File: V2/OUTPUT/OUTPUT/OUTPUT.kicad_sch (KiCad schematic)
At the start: 32 parts, among them J1 Conn_01x03, J2 Conn_01x03, J3 Conn_01x03, J4 Conn_01x03, J5 Conn_01x03, J6 Conn_01x03, J7 Conn_01x03, J8 Conn_01x03, Q1 QM6006D, Q2 QM6006D, Q3 QM6006D, Q4 QM6006D, Q5 QM6006D, Q6 QM6006D, Q7 QM6006D, Q8 QM6006D

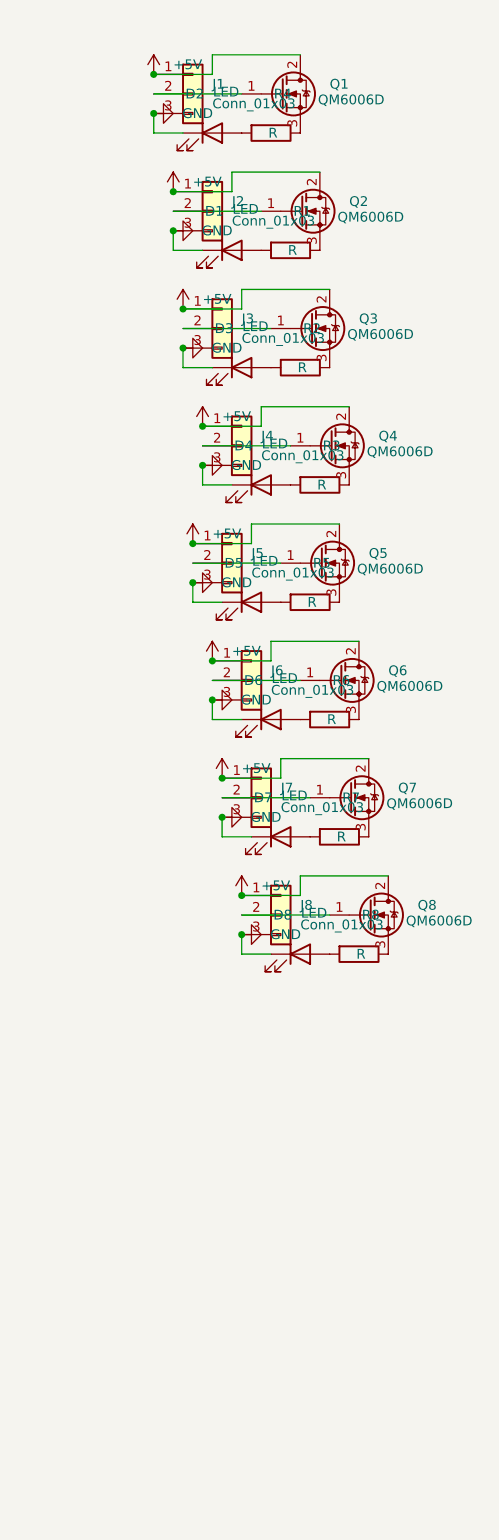
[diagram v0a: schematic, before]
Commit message: Auto-update: 28.03.2026 23:45:51,95
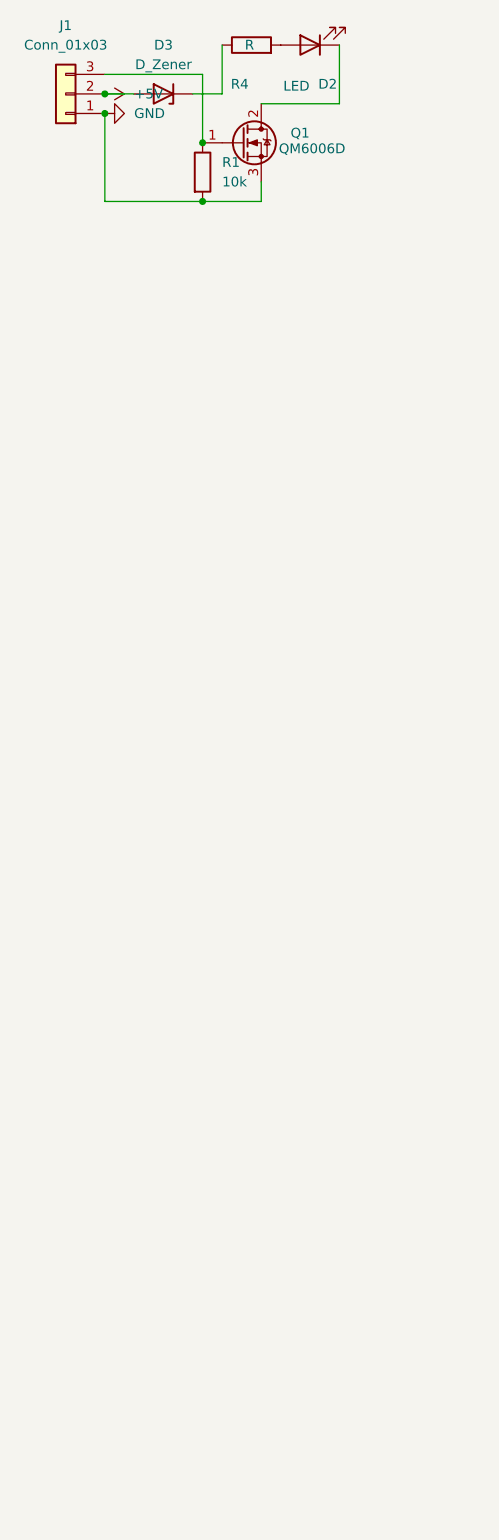
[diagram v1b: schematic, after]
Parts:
- removed D1, D3, D4, D5, D6, D7, D8: LED, LED_SMD:LED_1206_3216Metric, symbol Device:LED
- removed J2, J3, J4, J5, J6, J7, J8: Conn_01x03, Connector_PinSocket_2.54mm:PinSocket_1x03_P2.54mm_Horizontal, symbol Connector_Generic:Conn_01x03
- removed Q2, Q3, Q4, Q5, Q6, Q7, Q8: QM6006D, Package_TO_SOT_SMD:TO-252-2, symbol Transistor_FET:QM6006D
- removed R2, R3, R5, R6, R7, R8: R, Resistor_SMD:R_1206_3216Metric, symbol Device:R
- added D3: D_Zener, Diode_SMD:D_0201_0603Metric, symbol Device:D_Zener
- R1: value R -> 10k; footprint Resistor_SMD:R_1206_3216Metric -> (none)
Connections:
- net +5V: now also J1.2 (Pin_2), D3.2 (A); no longer J1.1 (Pin_1), Q1.2 (D)
- net GND: now also J1.1 (Pin_1), Q1.3 (S), R1.2; no longer D2.1 (K), J1.3 (Pin_3)
- net at R1.1: now also J1.3 (Pin_3), Q1.1 (G)
- net at R4.1: now also D3.1 (K); no longer Q1.3 (S)
- new net: D2.1 (K), Q1.2 (D)
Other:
- moved on the sheet: D2, J1, Q1, R4

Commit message: Auto-update: 29.03.2026  0:17:51,75
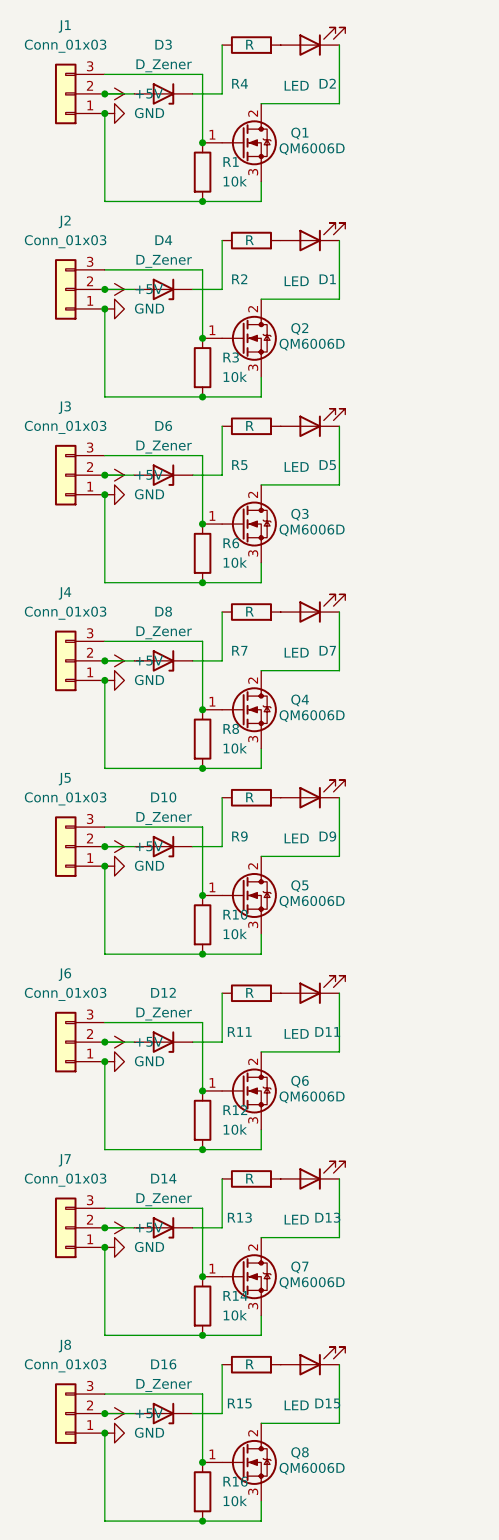
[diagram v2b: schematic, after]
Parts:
- added D1, D11, D13, D15, D5, D7, D9: LED, LED_SMD:LED_1206_3216Metric, symbol Device:LED
- added D10, D12, D14, D16, D4, D6, D8: D_Zener, Diode_SMD:D_0201_0603Metric, symbol Device:D_Zener
- added J2, J3, J4, J5, J6, J7, J8: Conn_01x03, Connector_PinSocket_2.54mm:PinSocket_1x03_P2.54mm_Horizontal, symbol Connector_Generic:Conn_01x03
- added Q2, Q3, Q4, Q5, Q6, Q7, Q8: QM6006D, Package_TO_SOT_SMD:SOT-23, symbol Transistor_FET:QM6006D
- added R10, R12, R14, R16, R3, R6, R8: 10k, Resistor_SMD:R_0201_0603Metric, symbol Device:R
- added R11, R13, R15, R2, R5, R7, R9: R, Resistor_SMD:R_0201_0603Metric, symbol Device:R
- Q1: footprint Package_TO_SOT_SMD:TO-252-2 -> Package_TO_SOT_SMD:SOT-23
- R1: footprint (none) -> Resistor_SMD:R_0201_0603Metric
- R4: footprint Resistor_SMD:R_1206_3216Metric -> Resistor_SMD:R_0201_0603Metric
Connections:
- net +5V: now also D10.2 (A), D12.2 (A), D14.2 (A), D16.2 (A), D4.2 (A), D6.2 (A), D8.2 (A), J2.2 (Pin_2), J3.2 (Pin_2), J4.2 (Pin_2), J5.2 (Pin_2), J6.2 (Pin_2), J7.2 (Pin_2), J8.2 (Pin_2)
- net GND: now also J2.1 (Pin_1), J3.1 (Pin_1), J4.1 (Pin_1), J5.1 (Pin_1), J6.1 (Pin_1), J7.1 (Pin_1), J8.1 (Pin_1), Q2.3 (S), Q3.3 (S), Q4.3 (S), Q5.3 (S), Q6.3 (S), Q7.3 (S), Q8.3 (S), R10.2, R12.2, R14.2, R16.2, R3.2, R6.2, R8.2
- new net: J2.3 (Pin_3), Q2.1 (G), R3.1
- new net: D1.1 (K), Q2.2 (D)
- new net: D1.2 (A), R2.2
- new net: J4.3 (Pin_3), Q4.1 (G), R8.1
- new net: J6.3 (Pin_3), Q6.1 (G), R12.1
- new net: D11.1 (K), Q6.2 (D)
- new net: D14.1 (K), R13.1
- new net: D5.1 (K), Q3.2 (D)
- new net: D5.2 (A), R5.2
- new net: J3.3 (Pin_3), Q3.1 (G), R6.1
- new net: J8.3 (Pin_3), Q8.1 (G), R16.1
- new net: D12.1 (K), R11.1
- new net: D11.2 (A), R11.2
- new net: D7.1 (K), Q4.2 (D)
- new net: D13.2 (A), R13.2
- new net: D8.1 (K), R7.1
- new net: D7.2 (A), R7.2
- new net: D15.1 (K), Q8.2 (D)
- new net: D10.1 (K), R9.1
- new net: D9.2 (A), R9.2
- new net: D9.1 (K), Q5.2 (D)
- new net: D6.1 (K), R5.1
- new net: J5.3 (Pin_3), Q5.1 (G), R10.1
- new net: D15.2 (A), R15.2
- new net: D16.1 (K), R15.1
- new net: J7.3 (Pin_3), Q7.1 (G), R14.1
- new net: D13.1 (K), Q7.2 (D)
- new net: D4.1 (K), R2.1
